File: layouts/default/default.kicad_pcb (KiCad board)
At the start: 2 copper layers, 48.5 x 77.2 mm, 90 parts

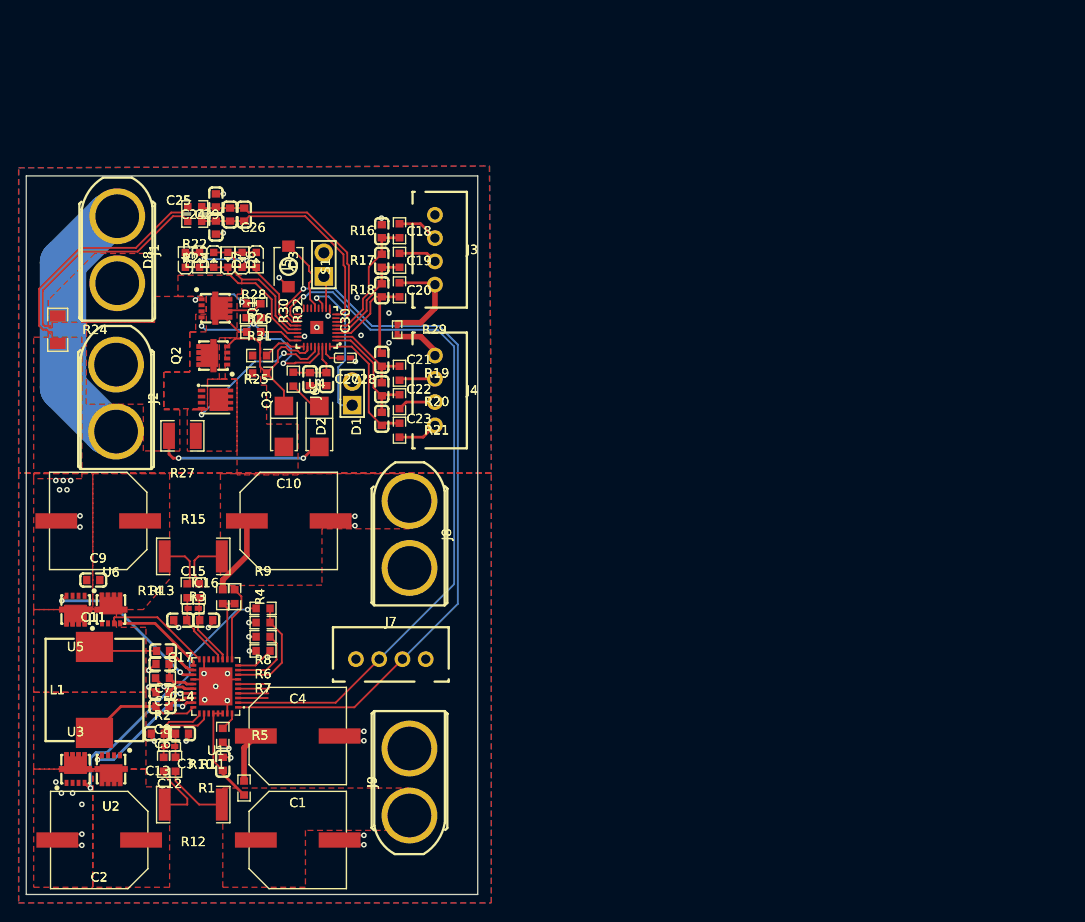
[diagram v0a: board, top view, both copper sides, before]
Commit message: What if 50x50 was enough?
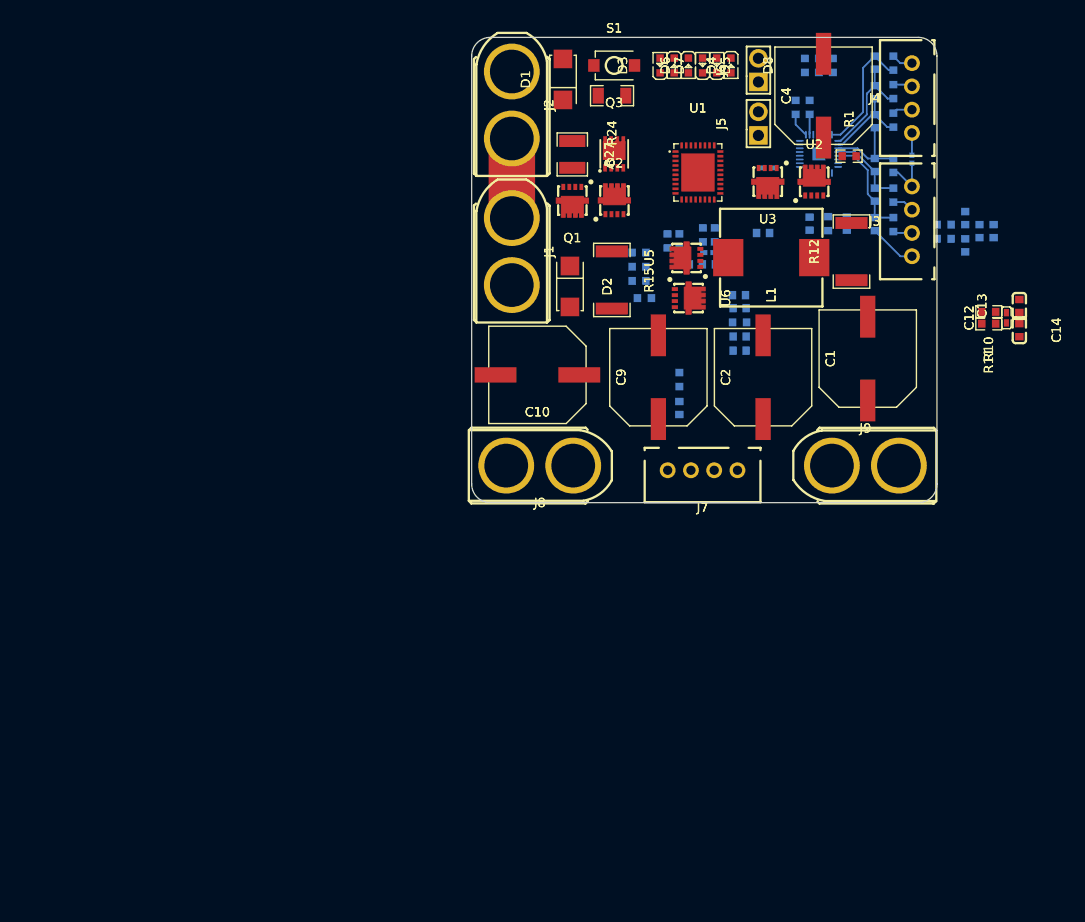
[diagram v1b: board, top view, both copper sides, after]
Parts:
- C11, C15, C16, C17, C18, C19, C20, C21, C22, C23, C24, C25, C26, C27, C28, C29, C3, C30, C5, C6, C7, C8, R13, R14, R16, R17, R18, R19, R2, R20, R21, R22, R23, R25, R26, R28, R29, R3, R30, R31, R32, R4, R5, R6, R7, R8, R9, U4: moved to B.Cu
- moved C13 103.4 mm to (206.5, 100.8), turned to 90 degrees
- moved R10 101.1 mm to (203.2, 101.5), turned to 180 degrees
- moved C12 101.0 mm to (205.2, 102.1), turned to 90 degrees
- moved C14 99.9 mm to (206.5, 103.5), turned to -90 degrees
- moved R11 99.4 mm to (203.2, 102.8), turned to 180 degrees
- moved U3 98.5 mm to (179.5, 86.8), turned to 180 degrees
- moved U2 97.5 mm to (184.5, 88.2), turned to 0 degrees
- moved R1 94.0 mm to (188.2, 84.8), turned to 0 degrees
- moved R12 92.4 mm to (188.5, 95.0), turned to 90 degrees
- moved C4 89.0 mm to (185.5, 78.2), turned to 90 degrees
- moved C2 87.0 mm to (179.0, 108.5), turned to 90 degrees
- moved L1 86.3 mm to (179.9, 95.7), turned to 180 degrees
- moved C11 81.1 mm to (179.0, 93.0), turned to 0 degrees
- moved C25 80.7 mm to (200.7, 94.3), turned to -90 degrees
- moved R22 80.6 mm to (198.5, 93.6)
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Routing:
- net SCL: track 80.3 -> 0.00 mm, vias 1 -> 0
- net SDA: track 76.4 -> 0.00 mm, vias 1 -> 0
- net -gnd: track 75.7 -> 0.00 mm, vias 35 -> 0
- net pack-gnd-0: track 31.9 -> 5.14 mm, vias 13 -> 0
- net pack-SRN: track 26.1 -> 0.00 mm
- net vbat: track 25.2 -> 0.00 mm, vias 4 -> 0
- net pack-SRP: track 24.5 -> 0.00 mm
- net CHG: track 21.1 -> 0.00 mm, vias 3 -> 0
- net pack-gnd-2: track 29.0 -> 8.55 mm
- net REGN: track 19.5 -> 0.00 mm, vias 2 -> 0
- net pack-anode: track 19.4 -> 0.00 mm, vias 2 -> 0
- net charger-D: track 18.5 -> 0.00 mm
- net -pos: track 18.2 -> 0.00 mm
- net charger-G-3: track 18.2 -> 0.00 mm, vias 2 -> 0
- net charger-G-2: track 18.0 -> 0.00 mm, vias 2 -> 0
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- added copper zone on In1.Cu, net -gnd
- removed copper zone on B.Cu, net -gnd
- removed copper zone on F.Cu, net -gnd
- removed copper zone on F.Cu, net -pos
- removed copper zone on F.Cu, net S
- removed copper zone on F.Cu, net charger-D
- removed copper zone on F.Cu, net charger-pos-0
- removed copper zone on F.Cu, net charger-pos-2
- removed copper zone on F.Cu, net pack-D-0
- removed copper zone on F.Cu, net pack-D-1
- removed copper zone on B.Cu, net pack-gnd-0
- removed copper zone on F.Cu, net pack-gnd-0
- removed copper zone on F.Cu, net vbat
- removed copper zone on F.Cu, net vsys
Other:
- board size 48.5 x 77.2 mm -> 50 x 50 mm
- copper layers 2 -> 4
